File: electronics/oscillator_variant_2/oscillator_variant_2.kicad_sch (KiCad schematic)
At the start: 56 parts, among them J1 module_2x15_left_input, J2 module_2x15_right_input, J3 Coax, Q1 BC817, U1 TL081, U2 NE5534, U3 TL082, U4 TL431, U5 NE5534

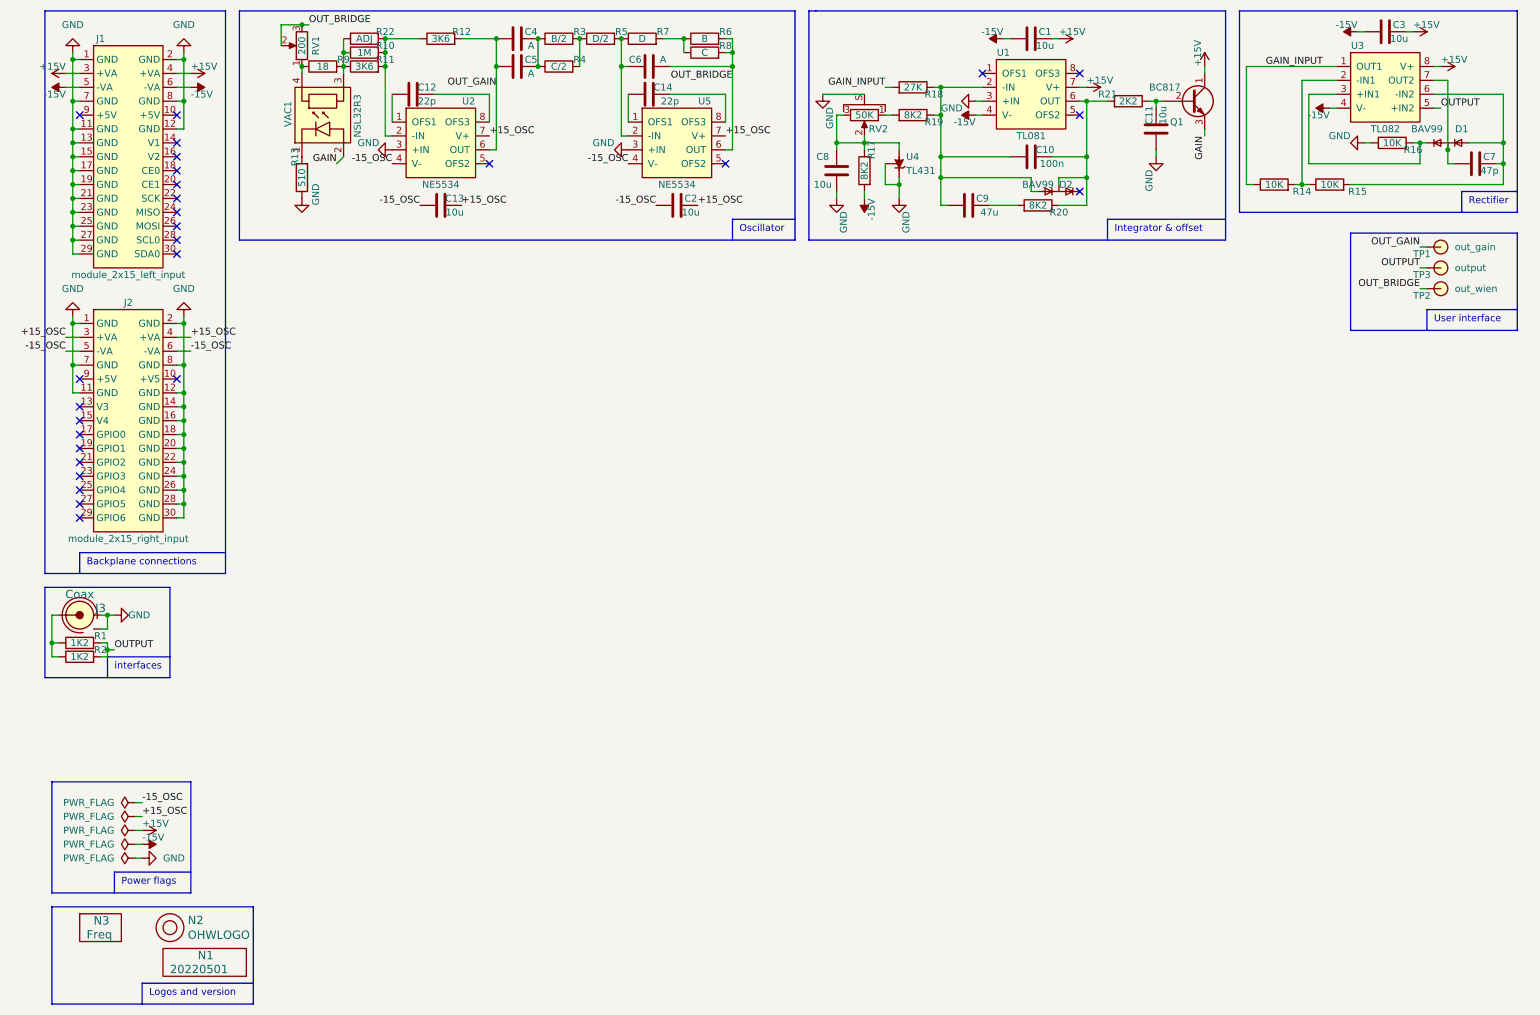
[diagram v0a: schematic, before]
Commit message: review completed
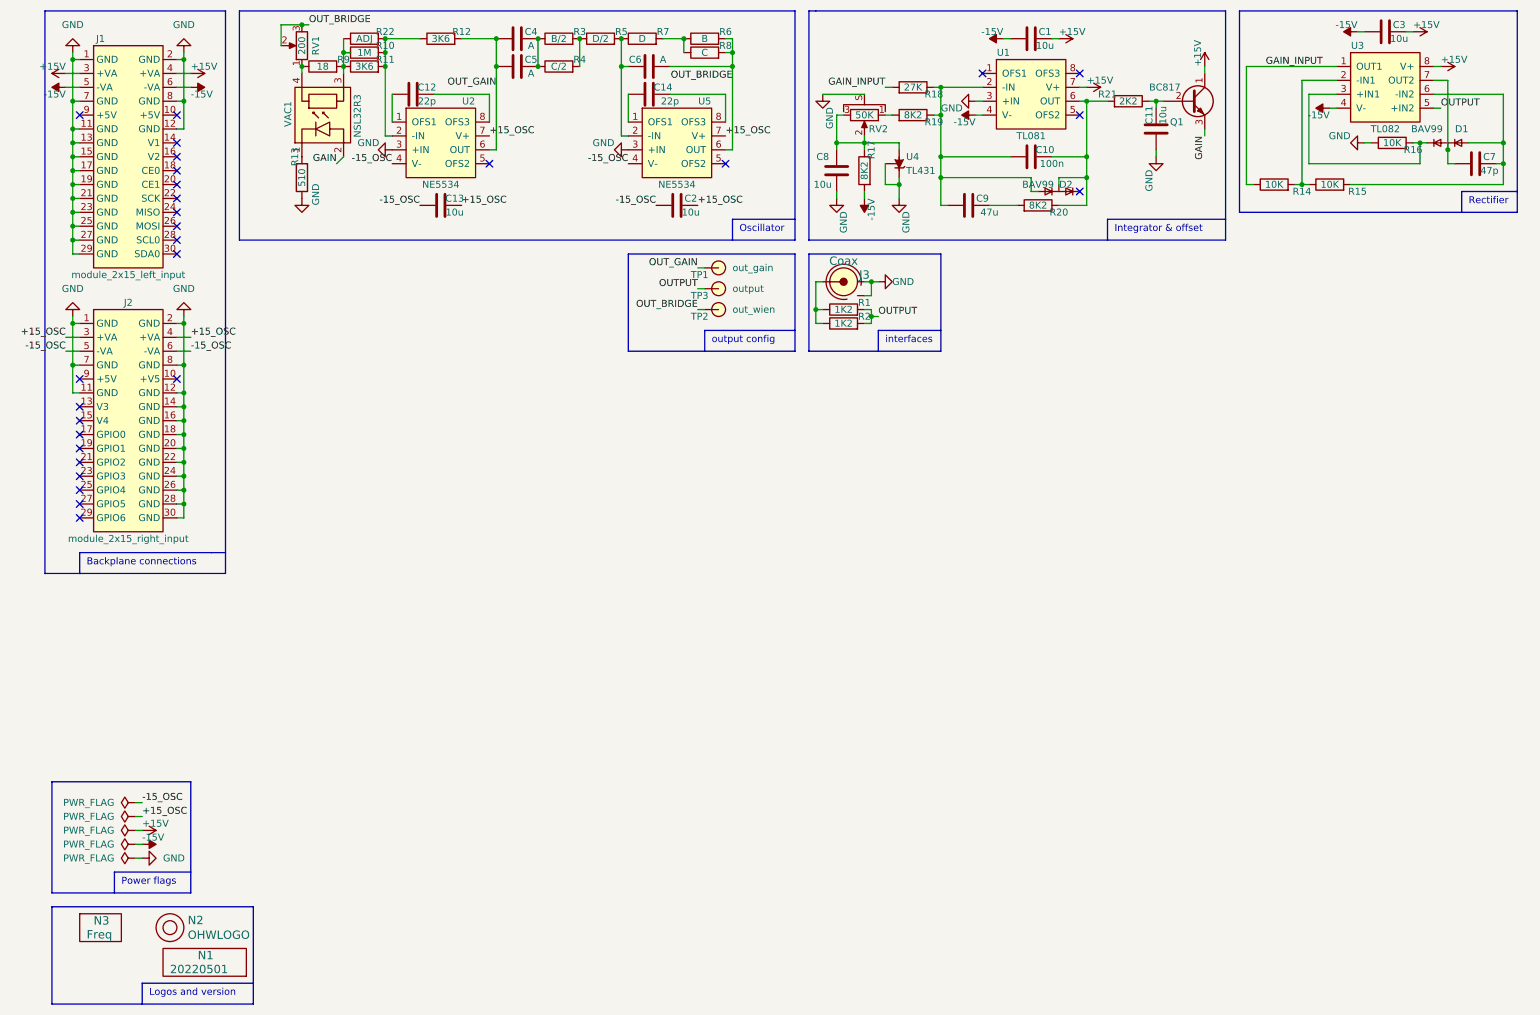
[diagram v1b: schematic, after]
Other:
- note added: "output config"
- note removed: "User interface"
- moved on the sheet: J3, R1, R2, TP1, TP2, TP3
